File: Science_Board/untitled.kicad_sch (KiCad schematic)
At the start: 8 parts, among them Q1 BS250, U1 AP63205WU

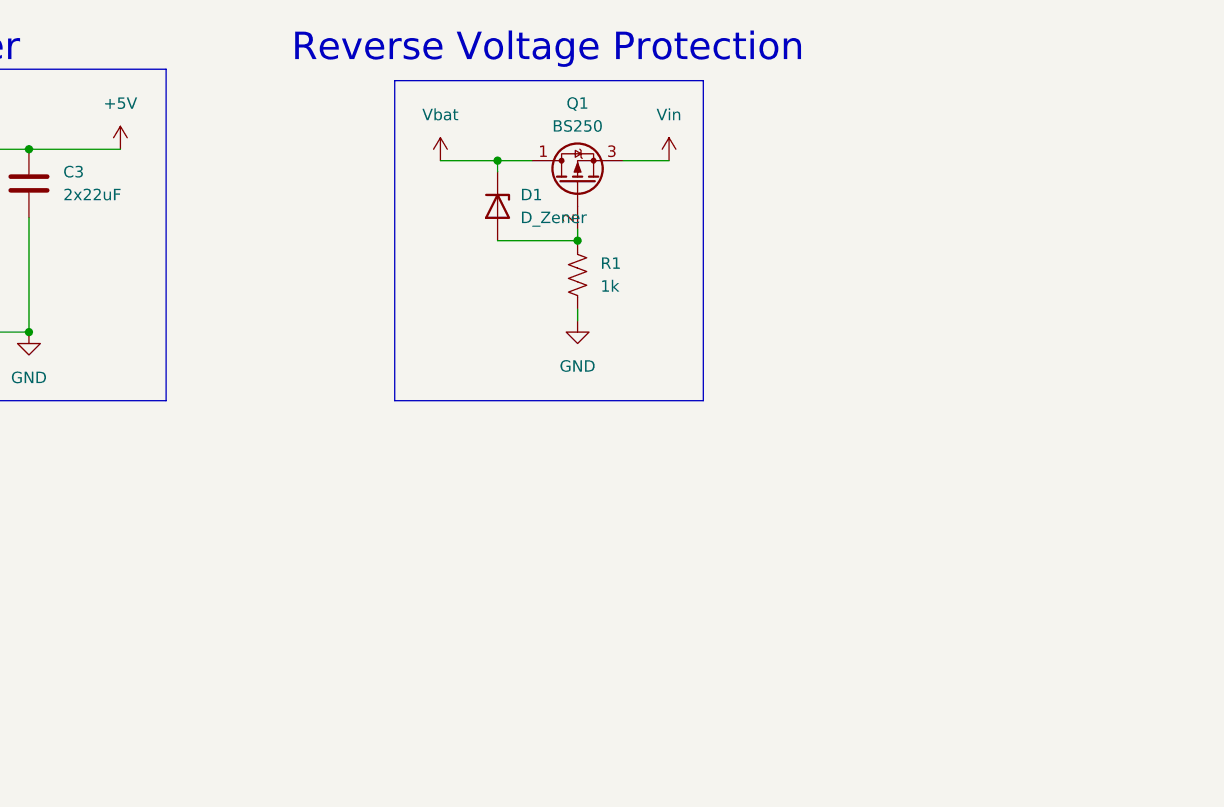
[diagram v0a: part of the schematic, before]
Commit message: RoveNode
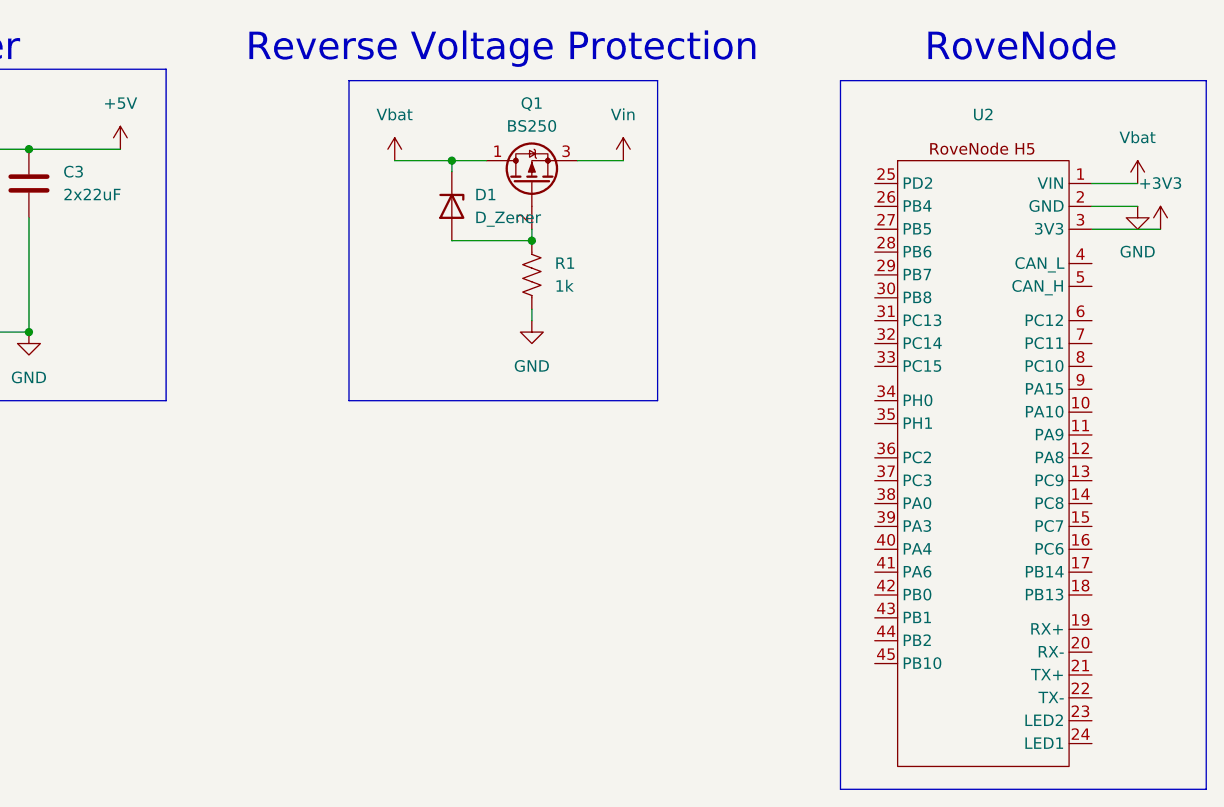
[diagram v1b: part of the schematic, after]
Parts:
- added U2: (no value), MRDT_Shields:RoveNode_H5, symbol MRDT_Shields:RoveNode_H5
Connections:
- net GND: now also U2.2 (GND)
- net Vbat: now also U2.1 (VIN)
- new net +3V3: U2.3 (3V3)
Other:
- note added: "RoveNode"
- moved on the sheet: D1, Q1, R1

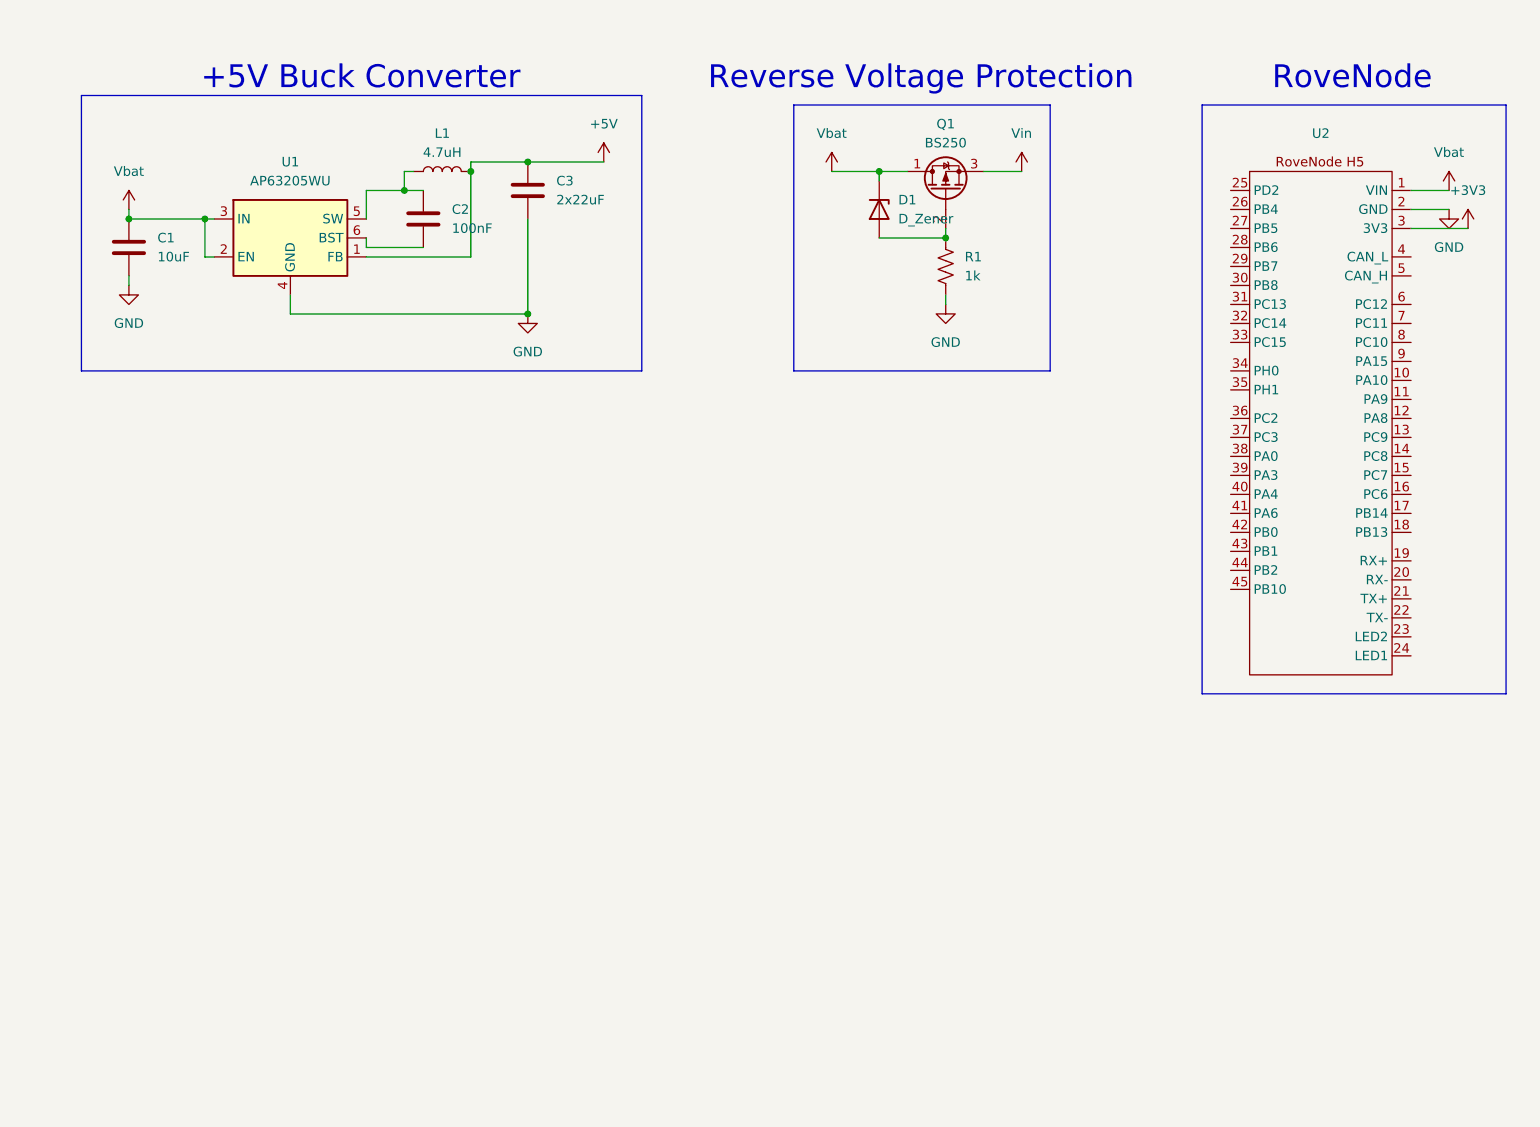
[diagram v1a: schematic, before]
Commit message: EFuses
They done
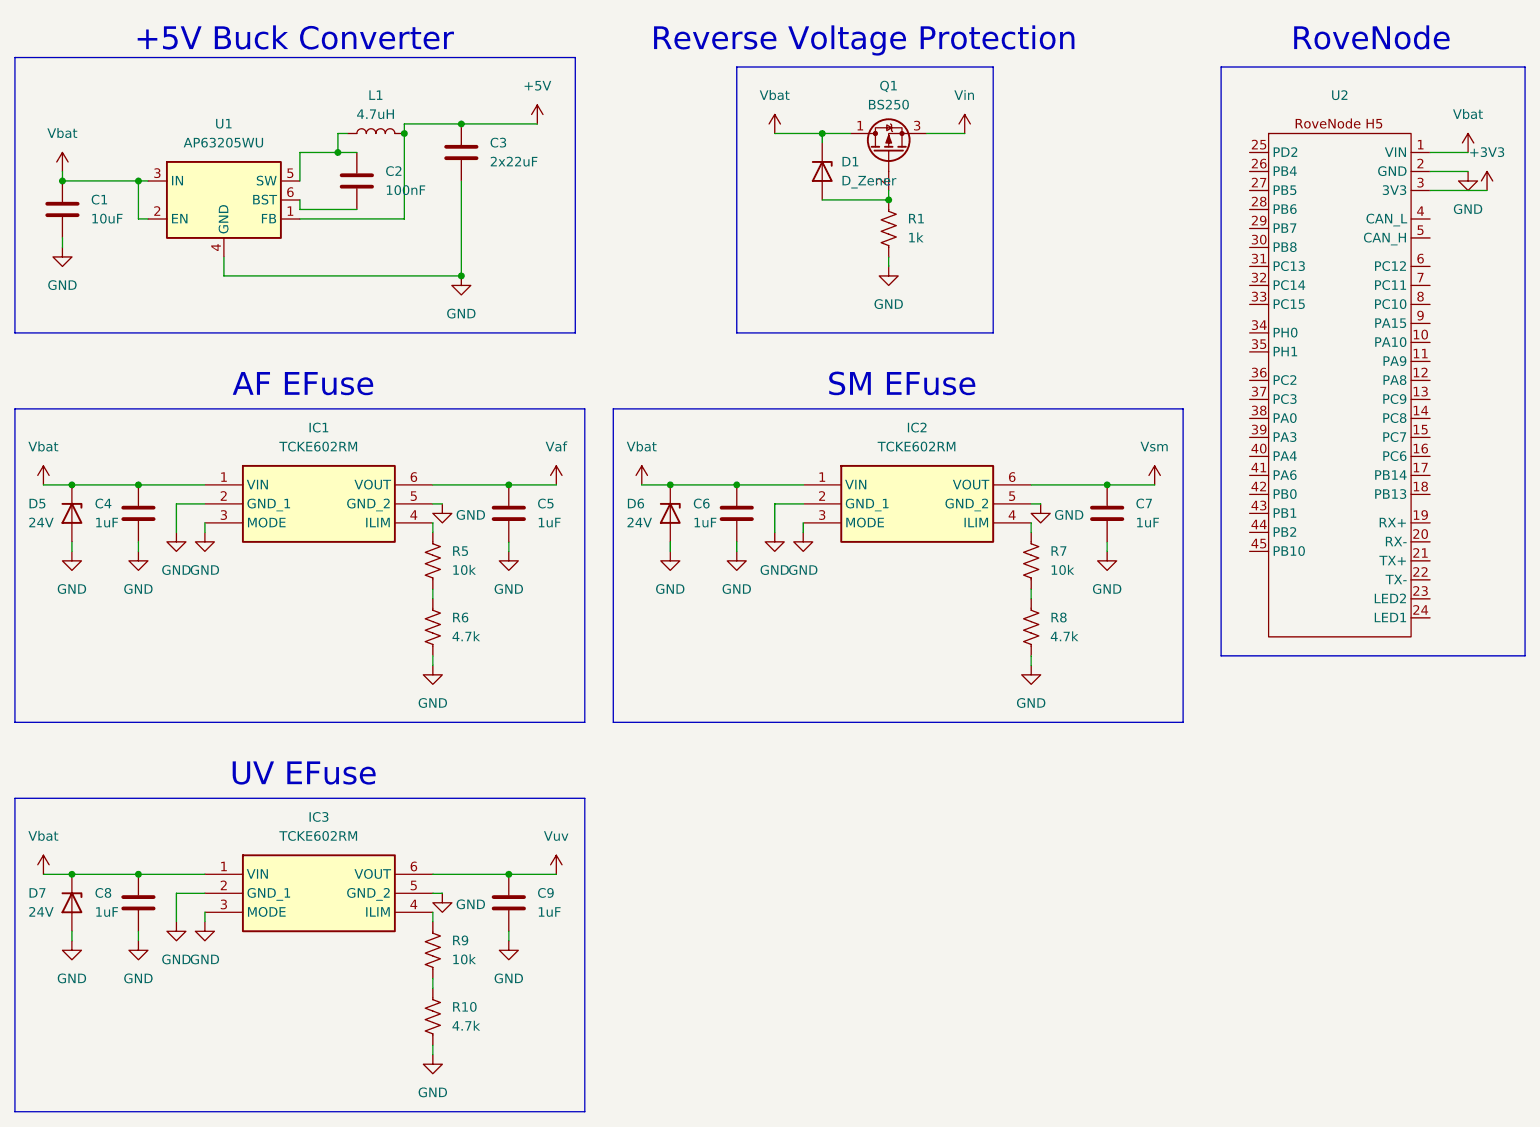
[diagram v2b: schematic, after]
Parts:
- added C4, C5, C6, C7, C8, C9: 1uF, symbol Device:C
- added D5, D6, D7: 24V, Package_DIP:DIP-40_W15.24mm, symbol Device:D_Zener
- added IC1, IC2, IC3: TCKE602RM, TCKE602RM, symbol MRDT_TCKE602RM:TCKE602RM
- added R10, R6, R8: 4.7k, Package_QFP:LQFP-100_14x14mm_P0.5mm, symbol Device:R_US
- added R5, R7, R9: 10k, symbol Device:R_US
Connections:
- net GND: now also C4.2, C5.2, C6.2, C7.2, C8.2, C9.2, D5.2 (A), D6.2 (A), D7.2 (A), IC1.2 (GND_1), IC1.3 (MODE), IC1.5 (GND_2), IC2.2 (GND_1), IC2.3 (MODE), IC2.5 (GND_2), IC3.2 (GND_1), IC3.3 (MODE), IC3.5 (GND_2), R10.2, R6.2, R8.2
- net Vbat: now also C4.1, C6.1, C8.1, D5.1 (K), D6.1 (K), D7.1 (K), IC1.1 (VIN), IC2.1 (VIN), IC3.1 (VIN)
- new net: R7.2, R8.1
- new net: IC3.4 (ILIM), R9.1
- new net: R10.1, R9.2
- new net: IC1.4 (ILIM), R5.1
- new net: IC2.4 (ILIM), R7.1
- new net: R5.2, R6.1
- new net Vaf: C5.1, IC1.6 (VOUT)
- new net Vsm: C7.1, IC2.6 (VOUT)
- new net Vuv: C9.1, IC3.6 (VOUT)
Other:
- note added: "AF EFuse"
- note added: "SM EFuse"
- note added: "UV EFuse"
- moved on the sheet: C1, C2, C3, D1, L1, Q1, R1, U1, U2
